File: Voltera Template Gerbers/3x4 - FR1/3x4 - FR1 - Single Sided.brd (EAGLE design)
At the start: 101.6 x 76.2 mm, 1 part

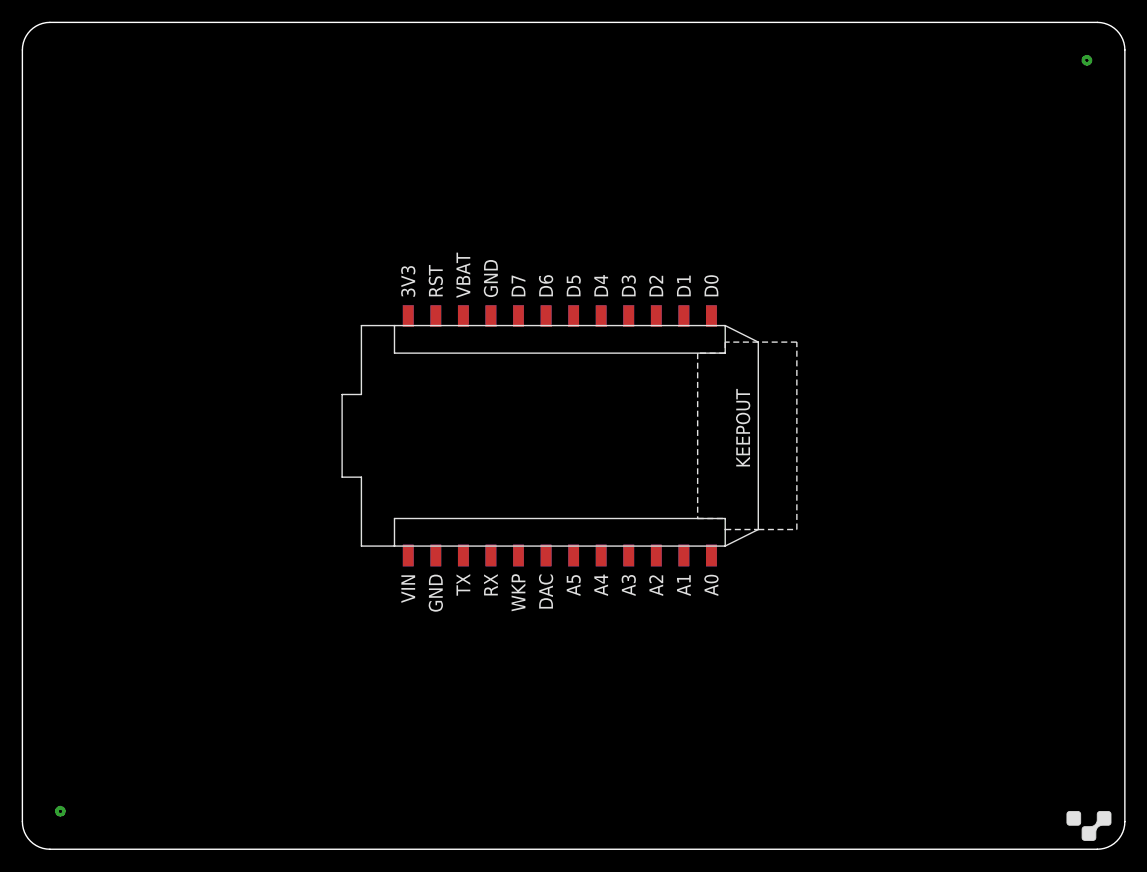
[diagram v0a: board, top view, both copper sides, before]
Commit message: Created FAB version for evertying, removed bad versions
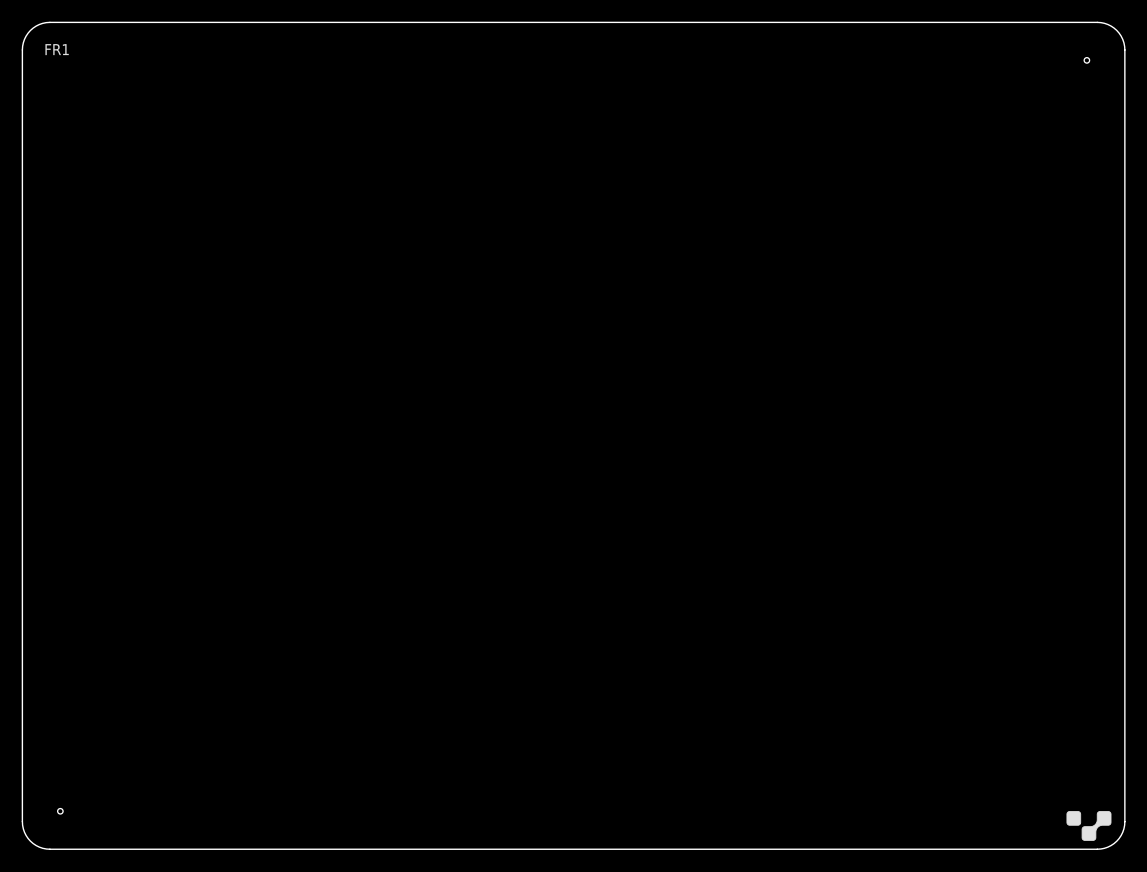
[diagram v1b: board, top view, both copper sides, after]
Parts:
- E$1: device voltera_community_lib:PHOTON -> voltera_EAGLE_community_lib:3X4_BOARD_FR1_RAW
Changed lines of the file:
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@@
 <?xml version="1.0" encoding="utf-8"?>
 <!DOCTYPE eagle SYSTEM "eagle.dtd">
-<eagle version="7.6.0">
+<eagle version="8.7.1">
 <drawing>
 <settings>
 <setting alwaysvectorfont="no"/>
+<setting keepoldvectorfont="yes"/>
 <setting verticaltext="up"/>
 </settings>
-<grid distance="0.05" unitdist="inch" unit="inch" style="lines" multiple="1" display="yes" altdistance="0.025" altunitdist="inch" altunit="inch"/>
+<grid distance="0.05" unitdist="inch" unit="inch" style="lines" multiple="1" display="no" altdistance="0.025" altunitdist="inch" altunit="inch"/>
 <layers>
 <layer number="1" name="Top" color="4" fill="1" visible="yes" active="yes"/>
@@
 <layer number="27" name="tValues" color="7" fill="1" visible="yes" active="yes"/>
 <layer number="28" name="bValues" color="7" fill="1" visible="yes" active="yes"/>
-<layer number="29" name="tStop" color="7" fill="3" visible="no" active="yes"/>
-<layer number="30" name="bStop" color="7" fill="6" visible="no" active="yes"/>
-<layer number="31" name="tCream" color="7" fill="4" visible="no" active="yes"/>
-<layer number="32" name="bCream" color="7" fill="5" visible="no" active="yes"/>
-<layer number="33" name="tFinish" color="6" fill="3" visible="no" active="yes"/>
-<layer number="34" name="bFinish" color="6" fill="6" visible="no" active="yes"/>
-<layer number="35" name="tGlue" color="7" fill="4" visible="no" active="yes"/>
-<layer number="36" name="bGlue" color="7" fill="5" visible="no" active="yes"/>
-<layer number="37" name="tTest" color="7" fill="1" visible="no" active="yes"/>
-<layer number="38" name="bTest" color="7" fill="1" visible="no" active="yes"/>
+<layer number="29" name="tStop" color="7" fill="3" visible="yes" active="yes"/>
+<layer number="30" name="bStop" color="7" fill="6" visible="yes" active="yes"/>
+<layer number="31" name="tCream" color="7" fill="4" visible="yes" active="yes"/>
+<layer number="32" name="bCream" color="7" fill="5" visible="yes" active="yes"/>
+<layer number="33" name="tFinish" color="6" fill="3" visible="yes" active="yes"/>
+<layer number="34" name="bFinish" color="6" fill="6" visible="yes" active="yes"/>
+<layer number="35" name="tGlue" color="7" fill="4" visible="yes" active="yes"/>
+<layer number="36" name="bGlue" color="7" fill="5" visible="yes" active="yes"/>
+<layer number="37" name="tTest" color="7" fill="1" visible="yes" active="yes"/>
+<layer number="38" name="bTest" color="7" fill="1" visible="yes" active="yes"/>
 <layer number="39" name="tKeepout" color="4" fill="11" visible="yes" active="yes"/>
 <layer number="40" name="bKeepout" color="1" fill="11" visible="yes" active="yes"/>
@@
 <layer number="42" name="bRestrict" color="1" fill="10" visible="yes" active="yes"/>
 <layer number="43" name="vRestrict" color="2" fill="10" visible="yes" active="yes"/>
-<layer number="44" name="Drills" color="7" fill="1" visible="no" active="yes"/>
-<layer number="45" name="Holes" color="7" fill="1" visible="no" active="yes"/>
-<layer number="46" name="Milling" color="3" fill="1" visible="no" active="yes"/>
-<layer number="47" name="Measures" color="7" fill="1" visible="no" active="yes"/>
+<layer number="44" name="Drills" color="7" fill="1" visible="yes" active="yes"/>
+<layer number="45" name="Holes" color="7" fill="1" visible="yes" active="yes"/>
+<layer number="46" name="Milling" color="3" fill="1" visible="yes" active="yes"/>
+<layer number="47" name="Measures" color="7" fill="1" visible="yes" active="yes"/>
 <layer number="48" name="Document" color="7" fill="1" visible="yes" active="yes"/>
 <layer number="49" name="Reference" color="7" fill="1" visible="yes" active="yes"/>
@@
 <param name="dpMaxLengthDifference" value="10mm"/>
 <param name="dpGapFactor" value="2.5"/>
-<param name="checkGrid" value="0"/>
 <param name="checkAngle" value="0"/>
 <param name="checkFont" value="1"/>
 <param name="checkRestrict" value="1"/>
+<param name="checkStop" value="0"/>
+<param name="checkValues" value="0"/>
 <param name="useDiameter" value="13"/>
 <param name="maxErrors" value="50"/>
@@
 <param name="TopRouterVariant" value="1"/>
 <param name="tpViaShape" value="round"/>
-<param name="PrefDir.1" value="a"/>
+<param name="PrefDir.1" value="|"/>
 <param name="PrefDir.2" value="0"/>
 <param name="PrefDir.3" value="0"/>
@@
 <param name="PrefDir.14" value="0"/>
 <param name="PrefDir.15" value="0"/>
-<param name="PrefDir.16" value="a"/>
+<param name="PrefDir.16" value="-"/>
 <param name="cfVia" value="8"/>
 <param name="cfNonPref" value="5"/>
@@
 </autorouter>
 <elements>
-<element name="E$1" library="voltera_community_lib" package="PHOTON" value="" x="0" y="0"/>
+<element name="E$1" library="voltera_EAGLE_community_lib" package="3X4_BOARD_FR1_RAW" value="" x="0" y="0"/>
 </elements>
 <signals>
